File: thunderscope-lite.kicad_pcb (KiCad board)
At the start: 2 copper layers, 275 parts, among them J1 BNC, J2 BNC, K1 UD2-4.5NUN-L, K2 UD2-4.5NUN-L, K3 UD2-4.5NUN-L, K4 UD2-4.5NUN-L, Q1 DMN62D0UW, Q2 DMN62D0UW, Q5 DMN62D0UW, Q6 DMN62D0UW, U1 ADA4930-2YCPZ-R2, U10 LMH6518, U11 NCP161ASN330T1G, U12 NCP161ASN330T1G, U13 LM27761, U14 REF2025, U15 OPA140AIDBVR, U2 AD9288BSTZ-40, U3 TMUX4053, U4 OPA140AIDBVR, U5 BUF802, U6 LMH6518, U7 TMUX4053, U8 OPA140AIDBVR, U9 BUF802

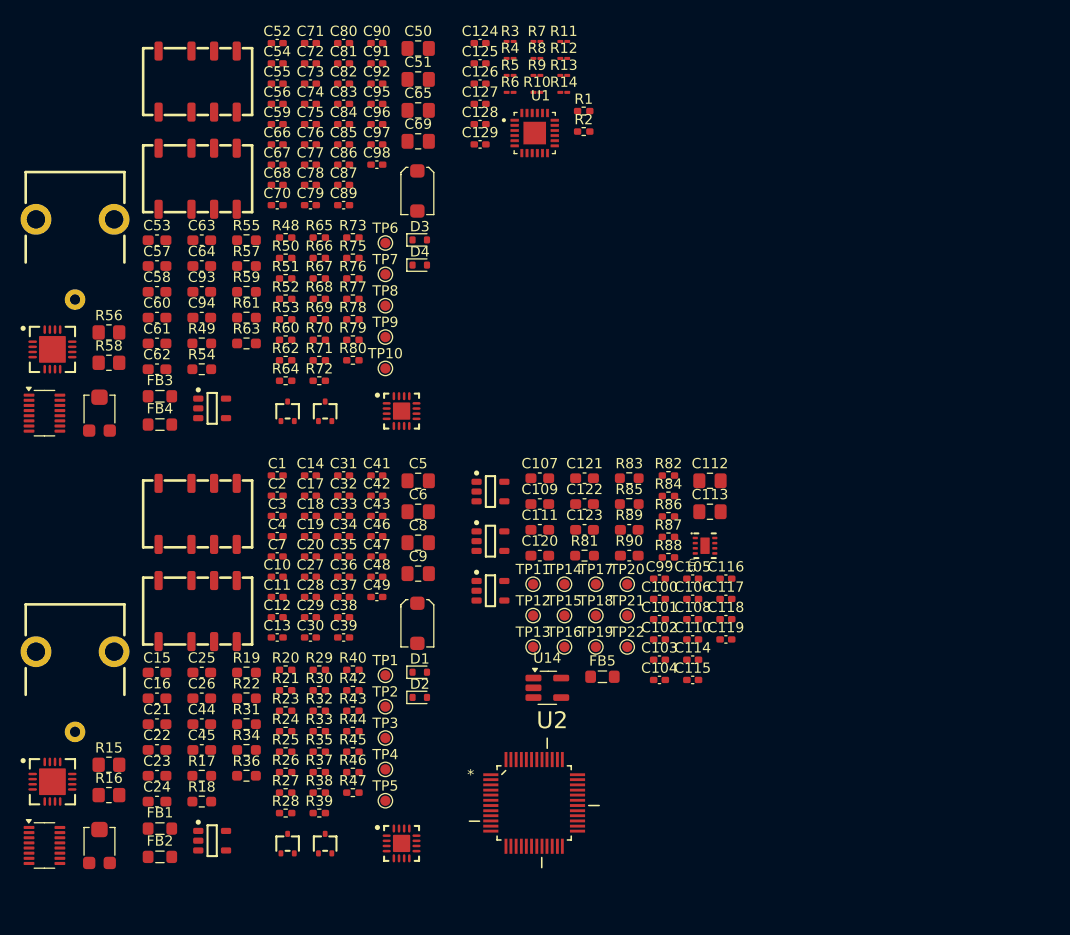
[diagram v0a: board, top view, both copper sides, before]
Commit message: updated a few stuff
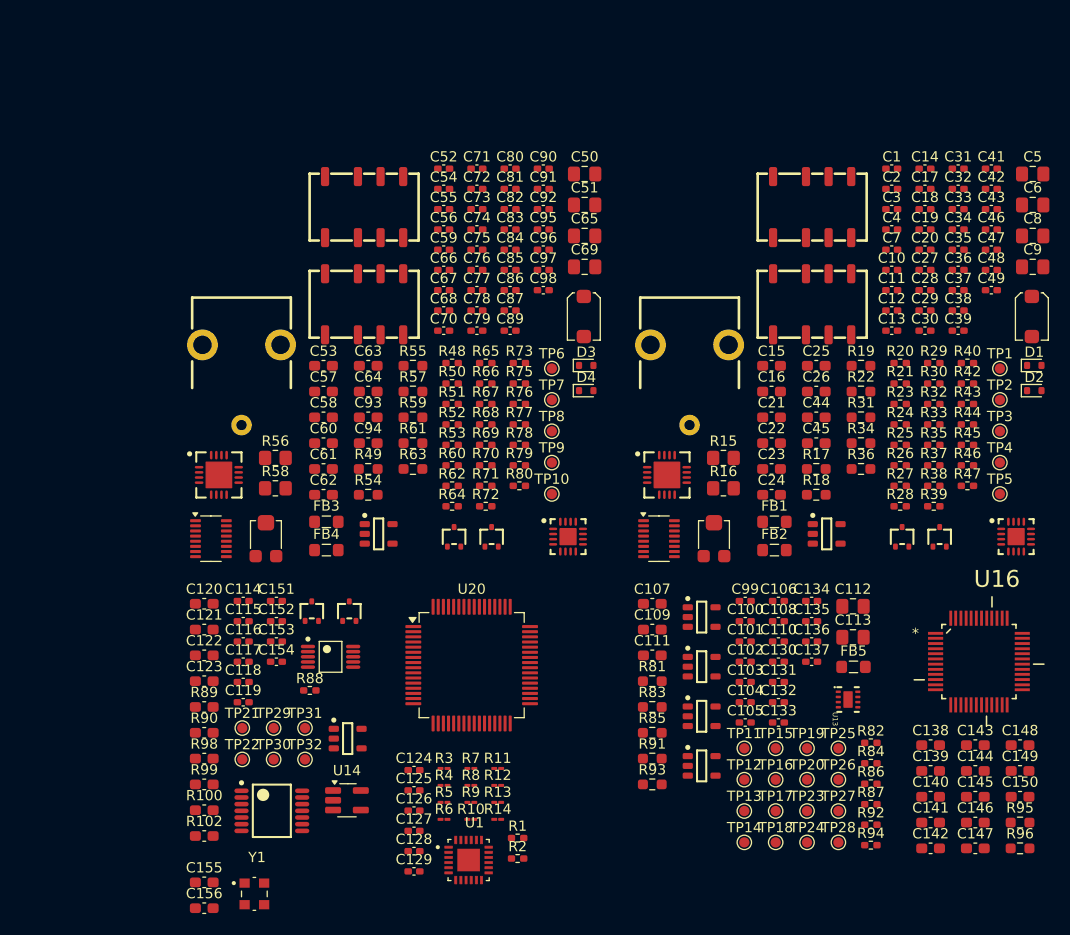
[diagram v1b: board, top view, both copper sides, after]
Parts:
- added C130: 10uF, Capacitor_SMD:C_0402_1005Metric_Pad0.74x0.62mm_HandSolder, F.Cu at (158.2, 100.0)
- added C131: 10uF, Capacitor_SMD:C_0402_1005Metric_Pad0.74x0.62mm_HandSolder, F.Cu at (158.2, 101.9)
- added C132: 1uF, Capacitor_SMD:C_0402_1005Metric_Pad0.74x0.62mm_HandSolder, F.Cu at (158.2, 103.9)
- added C133: 1uF, Capacitor_SMD:C_0402_1005Metric_Pad0.74x0.62mm_HandSolder, F.Cu at (158.2, 105.9)
- added C134: 10uF, Capacitor_SMD:C_0402_1005Metric_Pad0.74x0.62mm_HandSolder, F.Cu at (161.4, 94.0)
- added C135: 10uF, Capacitor_SMD:C_0402_1005Metric_Pad0.74x0.62mm_HandSolder, F.Cu at (161.4, 96.0)
- added C136: 1uF, Capacitor_SMD:C_0402_1005Metric_Pad0.74x0.62mm_HandSolder, F.Cu at (161.4, 98.0)
- added C137: 1uF, Capacitor_SMD:C_0402_1005Metric_Pad0.74x0.62mm_HandSolder, F.Cu at (161.4, 100.0)
- added C138: 100nF, Capacitor_SMD:C_0603_1608Metric_Pad1.08x0.95mm_HandSolder, F.Cu at (173.0, 108.1)
- added C139: 100nF, Capacitor_SMD:C_0603_1608Metric_Pad1.08x0.95mm_HandSolder, F.Cu at (173.0, 110.6)
- added C140: 100nF, Capacitor_SMD:C_0603_1608Metric_Pad1.08x0.95mm_HandSolder, F.Cu at (173.0, 113.1)
- added C141: 10uF, Capacitor_SMD:C_0603_1608Metric_Pad1.08x0.95mm_HandSolder, F.Cu at (173.0, 115.6)
- added C142: 10uF, Capacitor_SMD:C_0603_1608Metric_Pad1.08x0.95mm_HandSolder, F.Cu at (173.0, 118.1)
- added C143: 100nF, Capacitor_SMD:C_0603_1608Metric_Pad1.08x0.95mm_HandSolder, F.Cu at (177.4, 108.1)
- added C144: 100nF, Capacitor_SMD:C_0603_1608Metric_Pad1.08x0.95mm_HandSolder, F.Cu at (177.4, 110.6)
- added C145: 100nF, Capacitor_SMD:C_0603_1608Metric_Pad1.08x0.95mm_HandSolder, F.Cu at (177.4, 113.1)
- added C146: 100nF, Capacitor_SMD:C_0603_1608Metric_Pad1.08x0.95mm_HandSolder, F.Cu at (177.4, 115.6)
- added C147: 100nF, Capacitor_SMD:C_0603_1608Metric_Pad1.08x0.95mm_HandSolder, F.Cu at (177.4, 118.1)
- added C148: 100nF, Capacitor_SMD:C_0603_1608Metric_Pad1.08x0.95mm_HandSolder, F.Cu at (181.7, 108.1)
- added C149: 100nF, Capacitor_SMD:C_0603_1608Metric_Pad1.08x0.95mm_HandSolder, F.Cu at (181.7, 110.6)
- added C150: 100nF, Capacitor_SMD:C_0603_1608Metric_Pad1.08x0.95mm_HandSolder, F.Cu at (181.7, 113.1)
- added C151: 10uF, Capacitor_SMD:C_0402_1005Metric_Pad0.74x0.62mm_HandSolder, F.Cu at (109.4, 94.0)
- added C152: 1uF, Capacitor_SMD:C_0402_1005Metric_Pad0.74x0.62mm_HandSolder, F.Cu at (109.4, 96.0)
- added C153: 10uF, Capacitor_SMD:C_0402_1005Metric_Pad0.74x0.62mm_HandSolder, F.Cu at (109.4, 98.0)
- added C154: 1uF, Capacitor_SMD:C_0402_1005Metric_Pad0.74x0.62mm_HandSolder, F.Cu at (109.4, 100.0)
- added C155: 0.1uF, Capacitor_SMD:C_0603_1608Metric_Pad1.08x0.95mm_HandSolder, F.Cu at (102.4, 121.4)
- added C156: 10uF, Capacitor_SMD:C_0603_1608Metric_Pad1.08x0.95mm_HandSolder, F.Cu at (102.4, 123.9)
- added Q3: DMN62D0UW, Thunderscope_Rev5:GEN_SOT_323, F.Cu at (112.8, 95.0)
- added Q4: DMN62D0UW, Thunderscope_Rev5:GEN_SOT_323, F.Cu at (116.5, 95.0)
- added R100: 4.7K, Capacitor_SMD:C_0603_1608Metric_Pad1.08x0.95mm_HandSolder, F.Cu at (102.4, 114.4)
- added R102: 4.7K, Capacitor_SMD:C_0603_1608Metric_Pad1.08x0.95mm_HandSolder, F.Cu at (102.4, 116.9)
- added R91: 0.01R, Resistor_SMD:R_0603_1608Metric_Pad0.98x0.95mm_HandSolder, F.Cu at (145.9, 109.4)
- added R92: 10K, Resistor_SMD:R_0402_1005Metric_Pad0.72x0.64mm_HandSolder, F.Cu at (167.2, 115.8)
- added R93: 0.01R, Resistor_SMD:R_0603_1608Metric_Pad0.98x0.95mm_HandSolder, F.Cu at (145.9, 111.9)
- added R94: 10K, Resistor_SMD:R_0402_1005Metric_Pad0.72x0.64mm_HandSolder, F.Cu at (167.2, 117.8)
- added R95: 23.2K, Resistor_SMD:R_0603_1608Metric_Pad0.98x0.95mm_HandSolder, F.Cu at (181.7, 115.6)
- added R96: 10K, Resistor_SMD:R_0603_1608Metric_Pad0.98x0.95mm_HandSolder, F.Cu at (181.7, 118.1)
- added R98: 4.7K, Capacitor_SMD:C_0603_1608Metric_Pad1.08x0.95mm_HandSolder, F.Cu at (102.4, 109.4)
- added R99: 4.7K, Capacitor_SMD:C_0603_1608Metric_Pad1.08x0.95mm_HandSolder, F.Cu at (102.4, 111.9)
- added TP23: TestPoint, TestPoint:TestPoint_Pad_D1.0mm, F.Cu at (161.0, 114.5)
- added TP24: TestPoint, TestPoint:TestPoint_Pad_D1.0mm, F.Cu at (161.0, 117.5)
- added TP25: TestPoint, TestPoint:TestPoint_Pad_D1.0mm, F.Cu at (164.0, 108.4)
- added TP26: TestPoint, TestPoint:TestPoint_Pad_D1.0mm, F.Cu at (164.0, 111.4)
- added TP27: TestPoint, TestPoint:TestPoint_Pad_D1.0mm, F.Cu at (164.0, 114.5)
- added TP28: TestPoint, TestPoint:TestPoint_Pad_D1.0mm, F.Cu at (164.0, 117.5)
- added TP29: TestPoint, TestPoint:TestPoint_Pad_D1.0mm, F.Cu at (109.1, 106.4)
- added TP30: TestPoint, TestPoint:TestPoint_Pad_D1.0mm, F.Cu at (109.1, 109.5)
- added TP31: TestPoint, TestPoint:TestPoint_Pad_D1.0mm, F.Cu at (112.2, 106.4)
- added TP32: TestPoint, TestPoint:TestPoint_Pad_D1.0mm, F.Cu at (112.2, 109.5)
- added U16: AD9218BSTZ-105, AD9218BSTZ-105:QFP50P900X900X160-48N, F.Cu at (177.7, 99.9)
- added U17: NCP161ASN330T1G, Thunderscope_Rev5:GEN_SOT23_5_950_2900X1600X1450, F.Cu at (150.7, 105.3)
- added U18: NCP161ASN330T1G, Thunderscope_Rev5:GEN_SOT23_5_950_2900X1600X1450, F.Cu at (150.7, 110.1)
- added U19: MCP4452-104E, Thunderscope_Rev5:MC_TSSOP14, F.Cu at (108.9, 114.5)
- added U20: STM32H562RGTx, Package_QFP:LQFP-64_10x10mm_P0.5mm, F.Cu at (128.4, 100.3)
- added Y1: ASEM1-100.000MHZ-LC-T, ASEM1-100.000MHZ-LC-T:XTAL_ASEM1-100.000MHZ-LC-T, F.Cu at (107.2, 122.5)
- U2: value AD9288BSTZ-40 -> MCP4728; footprint AD9288BSTZ-40:QFP50P900X900X160-48N -> Thunderscope_Rev5:MC_MSOP10_UN
- moved C124 71.0 mm to (122.8, 110.5)
- moved C125 71.0 mm to (122.8, 112.5)
- moved C126 71.0 mm to (122.8, 114.4)
- moved R1 71.0 mm to (132.8, 117.1)
- moved R10 71.0 mm to (128.3, 115.3)
- moved R11 71.0 mm to (130.9, 110.3)
- moved R13 71.0 mm to (130.9, 113.6)
- moved R14 71.0 mm to (130.9, 115.3)
- moved R3 71.0 mm to (125.7, 110.3)
- moved R5 71.0 mm to (125.7, 113.6)
- moved R6 71.0 mm to (125.7, 115.3)
- moved R7 71.0 mm to (128.3, 110.3)
- moved R9 71.0 mm to (128.3, 113.6)
- moved U1 71.0 mm to (128.1, 119.2)
- moved C127 71.0 mm to (122.8, 116.4)
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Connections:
- net /ADC_driver/IN1_N renamed /ADC driver/IN1_N
- net /ADC_driver/IN1_P renamed /ADC driver/IN1_P
- net /ADC_driver/IN2_N renamed /ADC driver/IN2_N
- net /ADC_driver/IN2_P renamed /ADC driver/IN2_P
- net /FE_channel/+VPGA renamed /CH1/+VPGA
- net /FE_channel/ATTEN renamed /CH1/ATTEN
- net /FE_channel/ATTEN_1X renamed /CH1/ATTEN_1X
- net /FE_channel/ATTEN_50X_IN renamed /CH1/ATTEN_50X_IN
- net /FE_channel/ATTEN_50X_OUT renamed /CH1/ATTEN_50X_OUT
- net /FE_channel/ATTEN_IN renamed /CH1/ATTEN_IN
- net /FE_channel/ATTEN_OUT renamed /CH1/ATTEN_OUT
- net /FE_channel/BNC_IN renamed /CH1/BNC_IN
- net /FE_channel/BUF_IN renamed /CH1/BUF_IN
- net /FE_channel/BUF_IN_AUX renamed /CH1/BUF_IN_AUX
- net /FE_channel/BUF_IN_BIAS renamed /CH1/BUF_IN_BIAS
- net /FE_channel/BUF_OUT renamed /CH1/BUF_OUT
- net /FE_channel/BUF_OUT_R renamed /CH1/BUF_OUT_R
- net /FE_channel/DC_CPL renamed /CH1/DC_CPL
- net /FE_channel/DC_FB renamed /CH1/DC_FB
- net /FE_channel/PGA_BIAS renamed /CH1/PGA_BIAS
- net /FE_channel/PGA_CSn renamed /CH1/PGA_CSn
- net /FE_channel/PGA_SCLK renamed /CH1/PGA_SCLK
- net /FE_channel/PGA_SDIO renamed /CH1/PGA_SDIO
- net /FE_channel/TERM renamed /CH1/TERM
- net /FE_channel/TERM_1M renamed /CH1/TERM_1M
- net /FE_channel/TERM_50Z renamed /CH1/TERM_50Z
- net /FE_channel/TERM_50Z_R renamed /CH1/TERM_50Z_R
- net /FE_channel/TRIM renamed /TRIM_1
- net /FE_channel1/+VPGA renamed /CH2/+VPGA
- net /FE_channel1/ATTEN renamed /CH2/ATTEN
- net /FE_channel1/ATTEN_1X renamed /CH2/ATTEN_1X
- net /FE_channel1/ATTEN_50X_IN renamed /CH2/ATTEN_50X_IN
- net /FE_channel1/ATTEN_50X_OUT renamed /CH2/ATTEN_50X_OUT
- net /FE_channel1/ATTEN_IN renamed /CH2/ATTEN_IN
- net /FE_channel1/ATTEN_OUT renamed /CH2/ATTEN_OUT
- net /FE_channel1/BNC_IN renamed /CH2/BNC_IN
- net /FE_channel1/BUF_IN renamed /CH2/BUF_IN
- net /FE_channel1/BUF_IN_AUX renamed /CH2/BUF_IN_AUX
- net /FE_channel1/BUF_IN_BIAS renamed /CH2/BUF_IN_BIAS
- net /FE_channel1/BUF_OUT renamed /CH2/BUF_OUT
- net /FE_channel1/BUF_OUT_R renamed /CH2/BUF_OUT_R
- net /FE_channel1/DC_CPL renamed /CH2/DC_CPL
- net /FE_channel1/DC_FB renamed /CH2/DC_FB
- net /FE_channel1/PGA_BIAS renamed /CH2/PGA_BIAS
- net /FE_channel1/PGA_CSn renamed /CH2/PGA_CSn
- net /FE_channel1/PGA_SCLK renamed /CH2/PGA_SCLK
- net /FE_channel1/PGA_SDIO renamed /CH2/PGA_SDIO
- net /FE_channel1/TERM renamed /CH2/TERM
- net /FE_channel1/TERM_1M renamed /CH2/TERM_1M
- net /FE_channel1/TERM_50Z renamed /CH2/TERM_50Z
- net /FE_channel1/TERM_50Z_R renamed /CH2/TERM_50Z_R
- net /FE_channel1/TRIM renamed /TRIM_2
- net /voltage_gen/+5V_R_CP renamed /ACQ and FE Voltage Regs/+5V_R_CP
- net /voltage_gen/ACQ_EN renamed /ACQ and FE Voltage Regs/ACQ_EN
- net /voltage_gen/FE_EN renamed /ACQ and FE Voltage Regs/FE_EN
- net /voltage_gen/PGA_EN renamed /ACQ and FE Voltage Regs/PGA_EN
- net /voltage_gen/US- renamed /Front End Trim and Bias/US-
- C105 pad 1: +3V3_PGA -> PGA
- C106 pad 1: +3V3_PGA -> PGA
- C124 pad 1: /ADC_driver/VCM2 -> /VCM
- C125 pad 1: /ADC_driver/VCM1 -> /VCM
- R11 pad 2: /ADC_driver/OUT1_N -> /ADC driver/OUT1_N
- R12 pad 2: /ADC_driver/OUT1_P -> /ADC driver/OUT1_P
- R13 pad 2: /ADC_driver/OUT2_N -> /ADC driver/OUT2_N
- R14 pad 2: /ADC_driver/OUT2_P -> /ADC driver/OUT2_P
- TP16 pad 1: +3V3_PGA -> PGA
- U1 pad 11: /ADC_driver/VCM2 -> /VCM
- U1 pad 17: /ADC_driver/VCM1 -> /VCM
- U10 pad 13: /FE_channel1/VCM -> /VCM
- U12 pad 5: +3V3_PGA -> PGA
- U2 pad 1: unconnected-(U2-GND_6-Pad1) -> +5V
- U2 pad 10: /ADC_driver/OUT2_N -> GND
- U2 pad 2: /ADC_driver/OUT1_P -> /Front End Trim and Bias/TRIM_SCL_5V
- U2 pad 3: /ADC_driver/OUT1_N -> /Front End Trim and Bias/TRIM_SDA_5V
- U2 pad 4: unconnected-(U2-DFS-Pad4) -> GND
- U2 pad 6: unconnected-(U2-REFOUT-Pad6) -> /Front End Trim and Bias/VOUT1
- U2 pad 7: unconnected-(U2-REFINB-Pad7) -> /Front End Trim and Bias/VOUT2
- U2 pad 8: unconnected-(U2-S1-Pad8) -> /Front End Trim and Bias/VOUT3
- U2 pad 9: unconnected-(U2-S2-Pad9) -> /Front End Trim and Bias/VOUT4
- U6 pad 13: /FE_channel/VCM -> /VCM
